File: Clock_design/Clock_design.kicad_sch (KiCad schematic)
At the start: 42 parts, among them J1 Conn_02x03_Odd_Even, J2 Power_inlet_vertical, J3 Conn_01x06, Q1 NPN_2N3904_SOT23, SW1 Omron_B3F_SPST, SW2 Omron_B3F_SPST, SW3 Omron_B3F_SPST, SW4 Omron_B3F_SPST, U1 ATmega328-PU, U2 DS1307_DIP-8, U3 L7805, Y1 Crystal_16MHz, Y2 Crystal_32768Hz

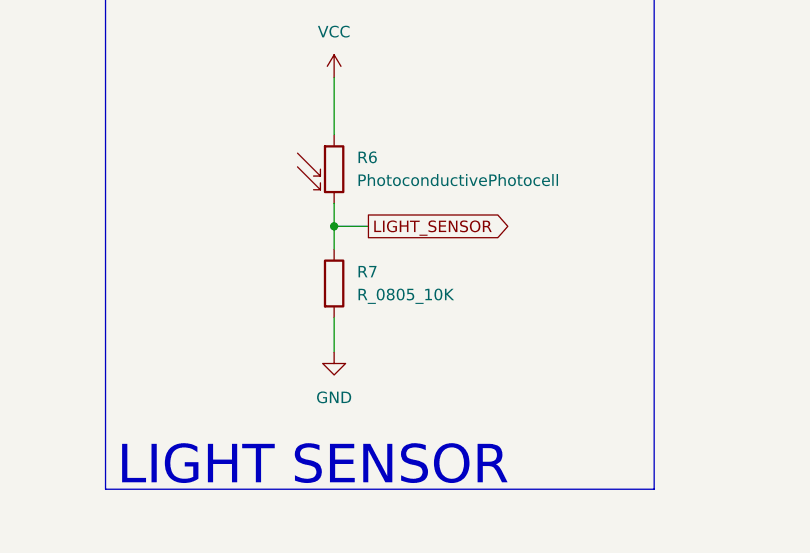
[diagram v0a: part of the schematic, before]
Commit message: Routing Update 3
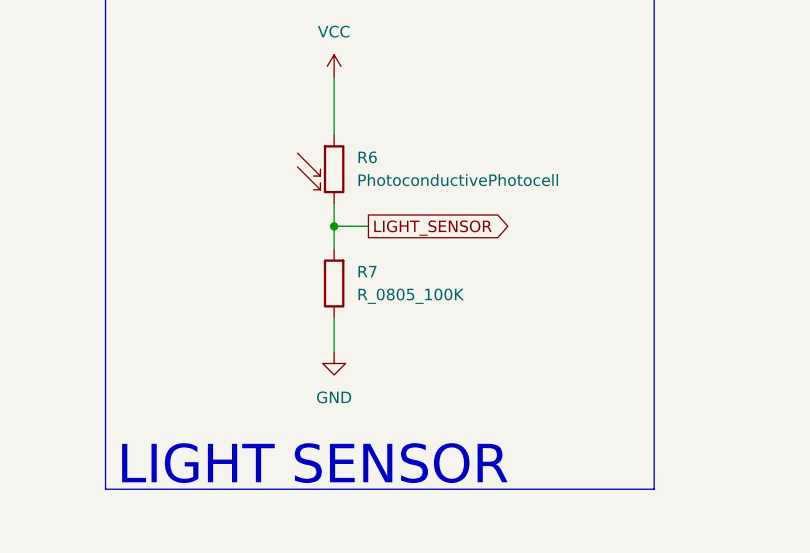
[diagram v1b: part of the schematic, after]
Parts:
- removed R7: R_0805_10K, footprints:R_0805_2012Metric, symbol HPS:R_0805_10K
- added R7: R_0805_100K, footprints:R_0805_2012Metric, symbol HPS:R_0805_100K
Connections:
- net GND: now also R7.1
- net LIGHT_SENSOR: now also R7.2
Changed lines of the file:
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@@
+    (pin "2")
+  )
+  (symbol (lib_id "HPS:R_0805_100K") (at 73.66 240.03 180) (unit 1)
+    (in_bom yes) (on_board yes) (fields_autoplaced)
+    (property "Reference" "R7" (id 0) (at 76.2 238.7599 0)
+      (effects (font (size 1.27 1.27)) (justify right))
+    )
+    (property "Value" "R_0805_100K" (id 1) (at 76.2 241.2999 0)
+      (effects (font (size 1.27 1.27)) (justify right))
+    )
+    (property "Footprint" "footprints:R_0805_2012Metric" (id 2) (at 73.66 223.52 0)
+      (effects (font (size 1.27 1.27)) hide)
+    )
+    (property "Datasheet" "https://www.digikey.com/en/products/detail/yageo/RC0805FR-07100KL/727544" (id 3) (at 76.2 240.03 0)
+      (effects (font (size 1.27 1.27)) hide)
+    )
+    (property "MFG" "Yageo" (id 4) (at 73.66 228.6 0)
+      (effects (font (size 1.27 1.27)) hide)
+    )
+    (property "MPN" "RC0805FR-07100KL" (id 5) (at 73.66 226.06 0)
+      (effects (font (size 1.27 1.27)) hide)
+    )
+    (property "Digikey PN" "311-100KCRCT-ND" (id 6) (at 73.66 220.98 0)
+      (effects (font (size 1.27 1.27)) hide)
+    )
+    (property "Mouser PN" "N/A" (id 7) (at 73.66 218.44 0)
+      (effects (font (size 1.27 1.27)) hide)
+    )
+    (property "Power" "N/A" (id 8) (at 73.66 215.9 0)
+      (effects (font (size 1.27 1.27)) hide)
+    )
+    (property "Tolerance" "N/A" (id 9) (at 73.66 213.36 0)
+      (effects (font (size 1.27 1.27)) hide)
+    )
+    (pin "1")
     (pin "2")
   )
@@
     )
     (property "MPN" "RC0805FR-071KL" (id 9) (at 91.44 173.99 0)
-      (effects (font (size 1.27 1.27)) hide)
-    )
-    (pin "1")
-    (pin "2")
-  )
-  (symbol (lib_id "HPS:R_0805_10K") (at 73.66 240.03 0) (unit 1)
-    (in_bom yes) (on_board yes) (fields_autoplaced)
-    (property "Reference" "R7" (id 0) (at 76.2 238.7599 0)
-      (effects (font (size 1.27 1.27)) (justify left))
-    )
-    (property "Value" "R_0805_10K" (id 1) (at 76.2 241.2999 0)
-      (effects (font (size 1.27 1.27)) (justify left))
-    )
-    (property "Footprint" "footprints:R_0805_2012Metric" (id 2) (at 73.66 256.54 0)
-      (effects (font (size 1.27 1.27)) hide)
-    )
-    (property "Datasheet" "https://www.digikey.com/en/products/detail/yageo/RC0805FR-0710KL/727535" (id 3) (at 71.12 240.03 0)
-      (effects (font (size 1.27 1.27)) hide)
-    )
-    (property "MFG" "Yageo" (id 4) (at 73.66 251.46 0)
-      (effects (font (size 1.27 1.27)) hide)
-    )
-    (property "MPN" "RC0805FR-0710KL" (id 5) (at 73.66 254 0)
-      (effects (font (size 1.27 1.27)) hide)
-    )
-    (property "Digikey PN" "311-10.0KCRCT-ND" (id 6) (at 73.66 259.08 0)
-      (effects (font (size 1.27 1.27)) hide)
-    )
-    (property "Mouser PN" "N/A" (id 7) (at 73.66 261.62 0)
-      (effects (font (size 1.27 1.27)) hide)
-    )
-    (property "Power" "N/A" (id 8) (at 73.66 264.16 0)
-      (effects (font (size 1.27 1.27)) hide)
-    )
-    (property "Tolerance" "N/A" (id 9) (at 73.66 266.7 0)
       (effects (font (size 1.27 1.27)) hide)
     )
@@
       (reference "R6") (unit 1) (value "PhotoconductivePhotocell") (footprint "footprints:R_LDR_4.9x4.2mm_P2.54mm_Vertical")
     )
-    (path "/5e6eada3-2f11-4981-9bd2-69d6f6375c6c"
-      (reference "R7") (unit 1) (value "R_0805_10K") (footprint "footprints:R_0805_2012Metric")
+    (path "/0bf32004-4913-4f13-884f-3ad0e36183c5"
+      (reference "R7") (unit 1) (value "R_0805_100K") (footprint "footprints:R_0805_2012Metric")
     )
     (path "/806ac943-a098-4def-bb09-8cc68e6a3938"
